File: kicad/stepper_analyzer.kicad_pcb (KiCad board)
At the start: 2 copper layers, 102 x 57 mm, 25 parts, among them J1 Connector_Conn_01x04_Male, J2 Connector_Conn_01x04_Male, M1 Motor, Q1 AO3400A, U1 (CURRENT SENSOR), U2 (CURRENT SENSOR), U3 Pico

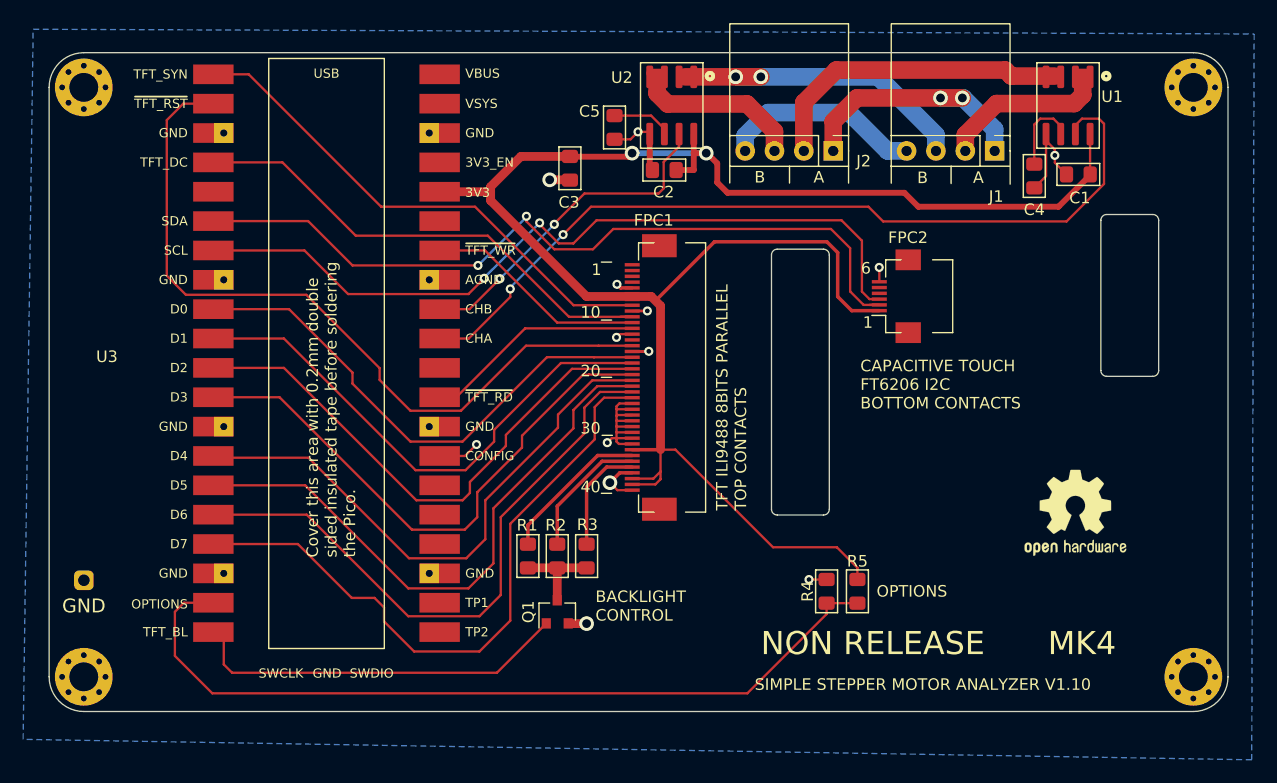
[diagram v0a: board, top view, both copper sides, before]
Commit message: Resoted Kicad files to V1.00 release.
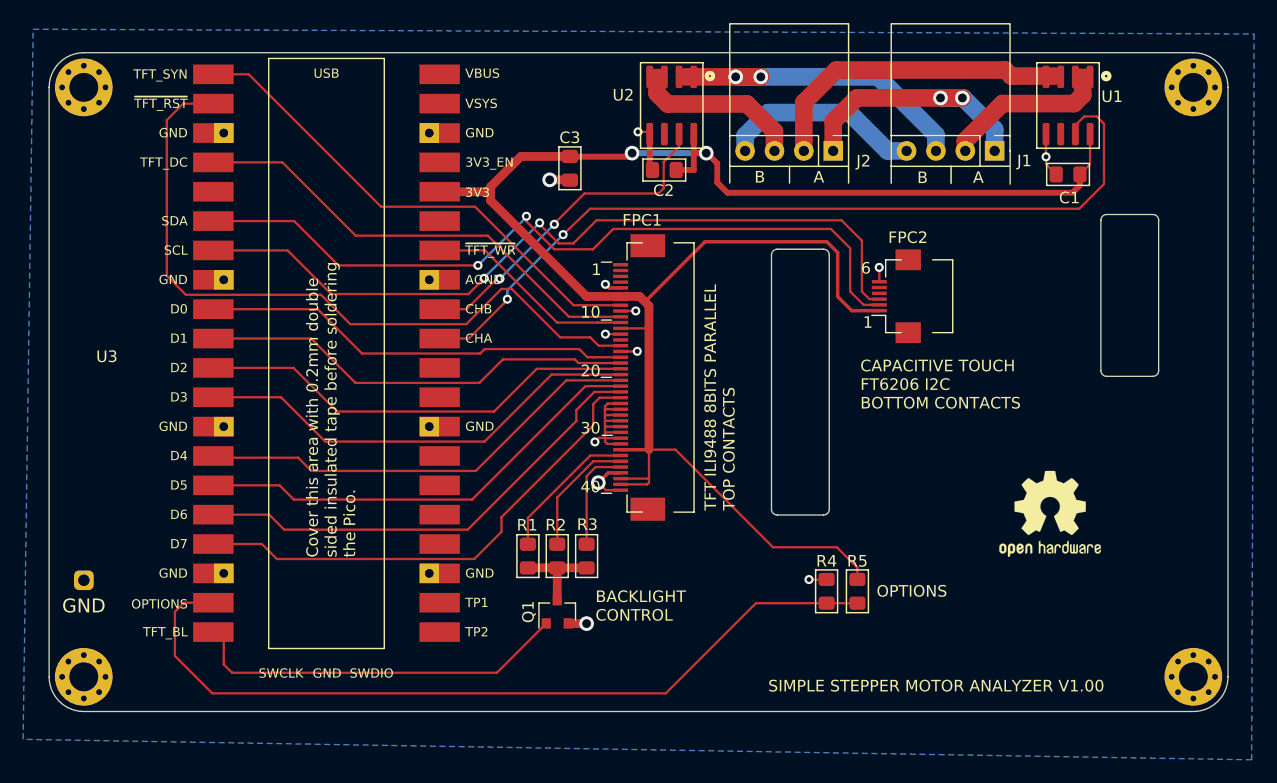
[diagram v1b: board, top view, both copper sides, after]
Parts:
- removed C4: 1nf, stepper_motor_analyzer:C_0805_2012Metric_Pad1.15x1.40mm_HandSolder
- removed C5: DNP, stepper_motor_analyzer:C_0805_2012Metric_Pad1.15x1.40mm_HandSolder
- R4: footprint stepper_motor_analyzer:R_0805_2012Metric_Pad1.15x1.40mm_HandSolder -> stepper_motor_analyzer:R_0805_2012Metric_Pad1.15x1.40mm_HandSolder_no_3d
- U1, U2: value (CURRENT SENSOR) -> ACS70331EOLCTR-2P5B3
- moved LOGO1 2.19 mm to (85.6, -17.1)
- moved FPC1 1.00 mm to (50.3, -28.9)
- moved C1 0.89 mm to (87.2, -46.5)
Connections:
- FPC1 pad 12: /~TFT_RD -> +3V3
- U3 pad 27: GND -> Net-(U3-Pad27)
- U3 pad 29: /~TFT_RD -> Net-(U3-Pad29)
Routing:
- net /~TFT_RD: track 20.3 -> 0.00 mm
- net GND: track 53.1 -> 39.3 mm, vias 13 -> 12
- net /D7: track 55.6 -> 42.5 mm
- net /D6: track 52.3 -> 40.4 mm
- net /D5: track 50.0 -> 38.9 mm
- net /D4: track 48.0 -> 38.1 mm
- net /D3: track 47.5 -> 38.3 mm
- net /D2: track 45.9 -> 37.4 mm
- net /D1: track 44.5 -> 36.9 mm
- net /D0: track 43.7 -> 36.4 mm
- net Net-(U1-Pad6): track 7.10 -> 0.00 mm
- net Net-(U2-Pad6): track 5.24 -> 0.00 mm
- net /~TFT_RST: track 67.0 -> 63.3 mm
- net +3V3: track 162.7 -> 165.2 mm
- net /TFT_DC: track 41.9 -> 39.9 mm
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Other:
- board text added: "SIMPLE STEPPER MOTOR ANALYZER V1.00"
- board text removed: "MK4"
- board text removed: "NON RELEASE"
- board text removed: "SIMPLE STEPPER MOTOR ANALYZER V1.10"
